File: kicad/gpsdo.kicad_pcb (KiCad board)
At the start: 2 copper layers, 76.2 x 30.5 mm, 32 parts, among them J1 Conn_Coaxial, J2 Conn_01x04_Male, J3 Conn_01x04_Male, J4 Conn_01x04_Male, J5 Conn_01x04_Male, J6 Conn_01x04_Male, U1 MSP430F5171IDA, U11 47L64, U2 MAX-8Q, U3 549CAAC000111BBG, U4 Si7051-A20

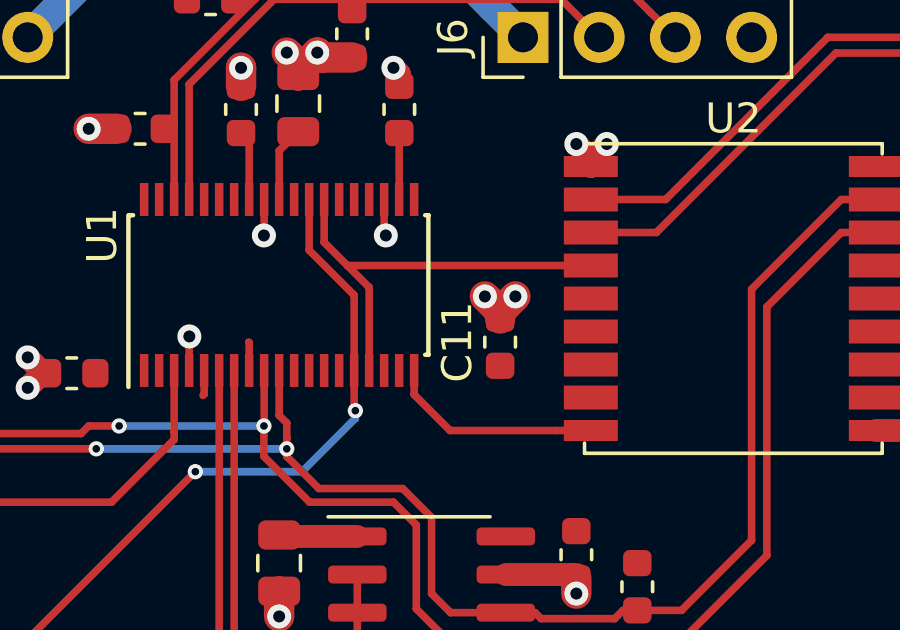
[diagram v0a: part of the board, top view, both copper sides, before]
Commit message: update pcb layout
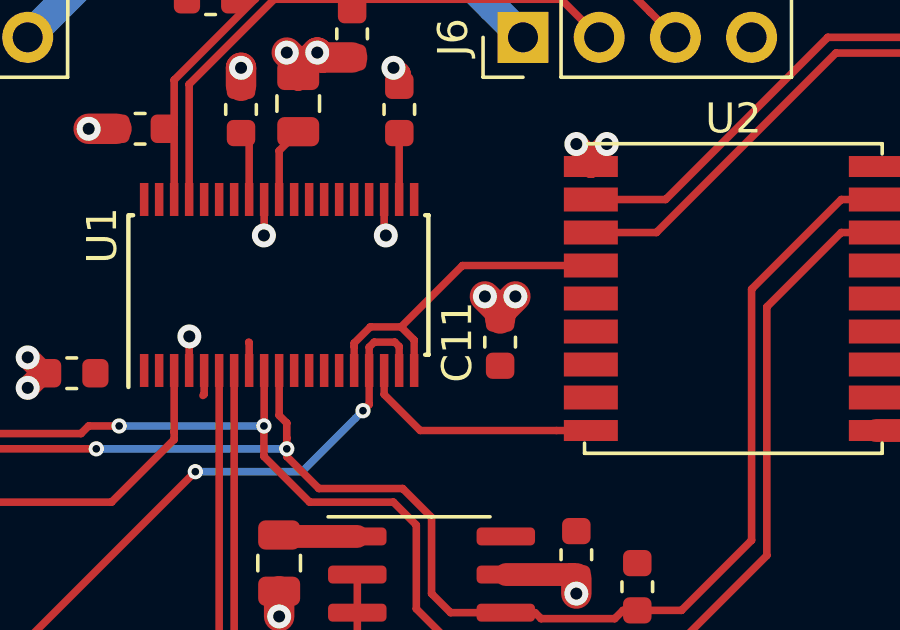
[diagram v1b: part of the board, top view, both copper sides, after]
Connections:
- U1 pad 15: PPS -> gPPS
- U1 pad 16: gPPS -> PPS
- U1 pad 17: +3V3 -> /gRST
- U1 pad 18: +3V3 -> PPS
- U1 pad 19: /gRST -> gPPS
- U1 pad 26: gPPS -> +3V3
- U1 pad 27: PPS -> +3V3
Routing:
- net PPS: track 27.2 -> 23.8 mm
- net gPPS: track 14.5 -> 11.5 mm
- net /gRST: track 7.19 -> 8.19 mm
